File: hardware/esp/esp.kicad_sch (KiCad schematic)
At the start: 34 parts, among them J1 USB_C_Receptacle_USB2.0_16P, J2 Conn_01x02, J3 USB_C_Receptacle_USB2.0_16P, J4 Conn_01x02, SW1 RESET, SW2 BOOT, U1 AMS1117-3.3, U2 ESP32-S3-WROOM-1, U6 CP2102N-Axx-xQFN20

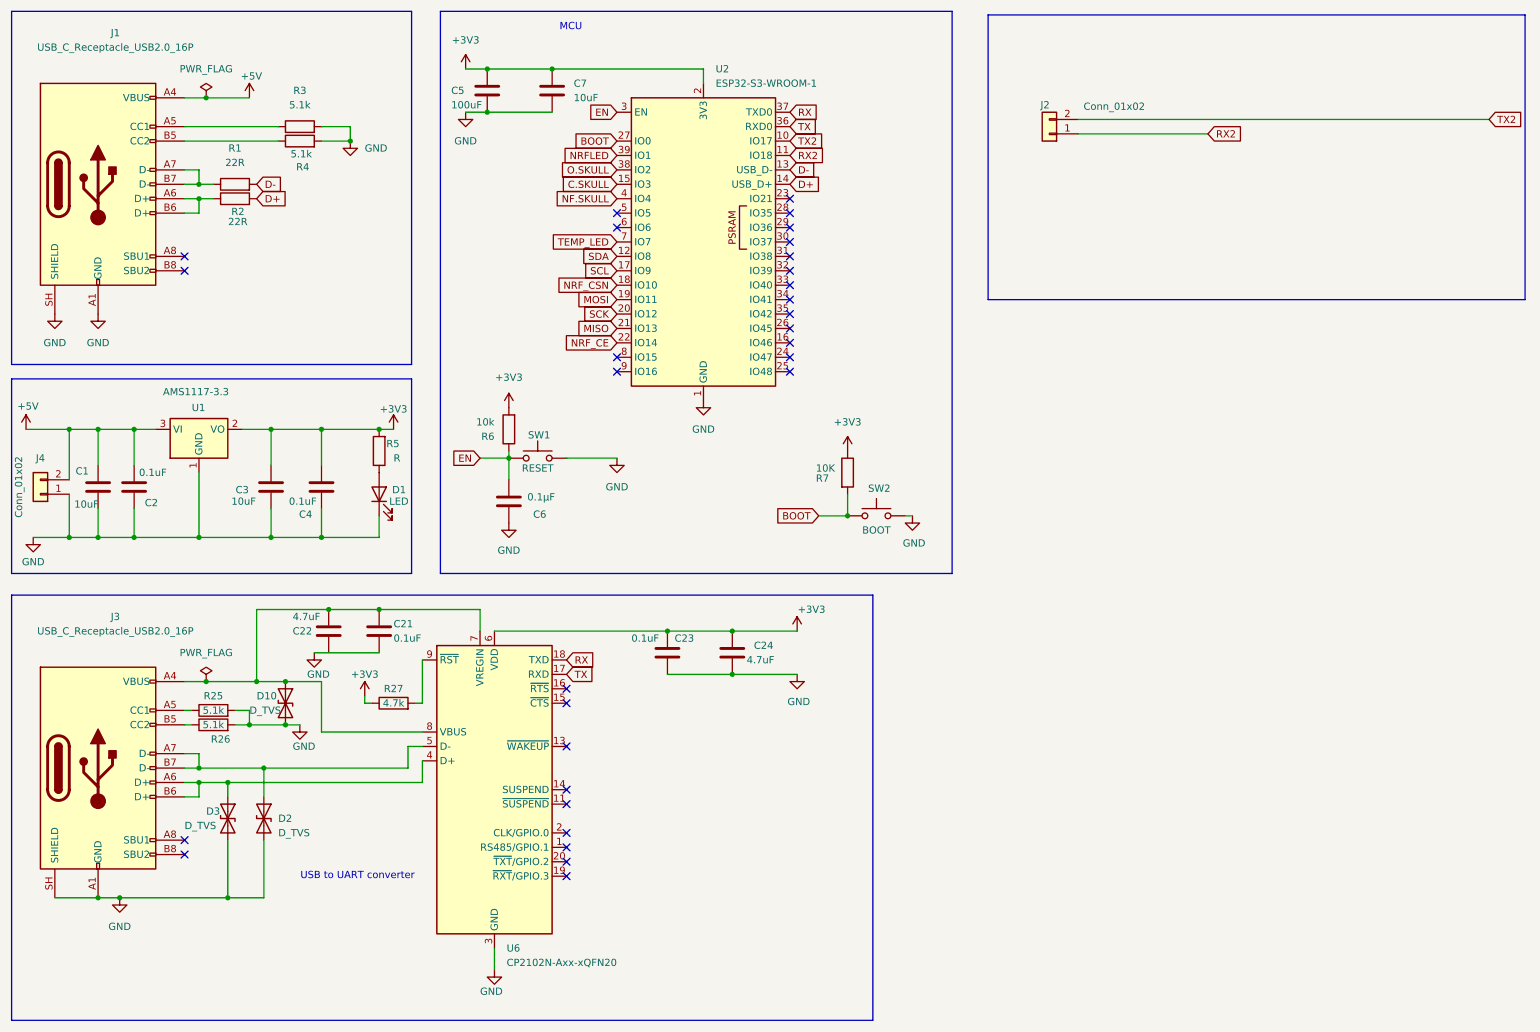
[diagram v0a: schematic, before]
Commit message: Updating pins, and scehmatic
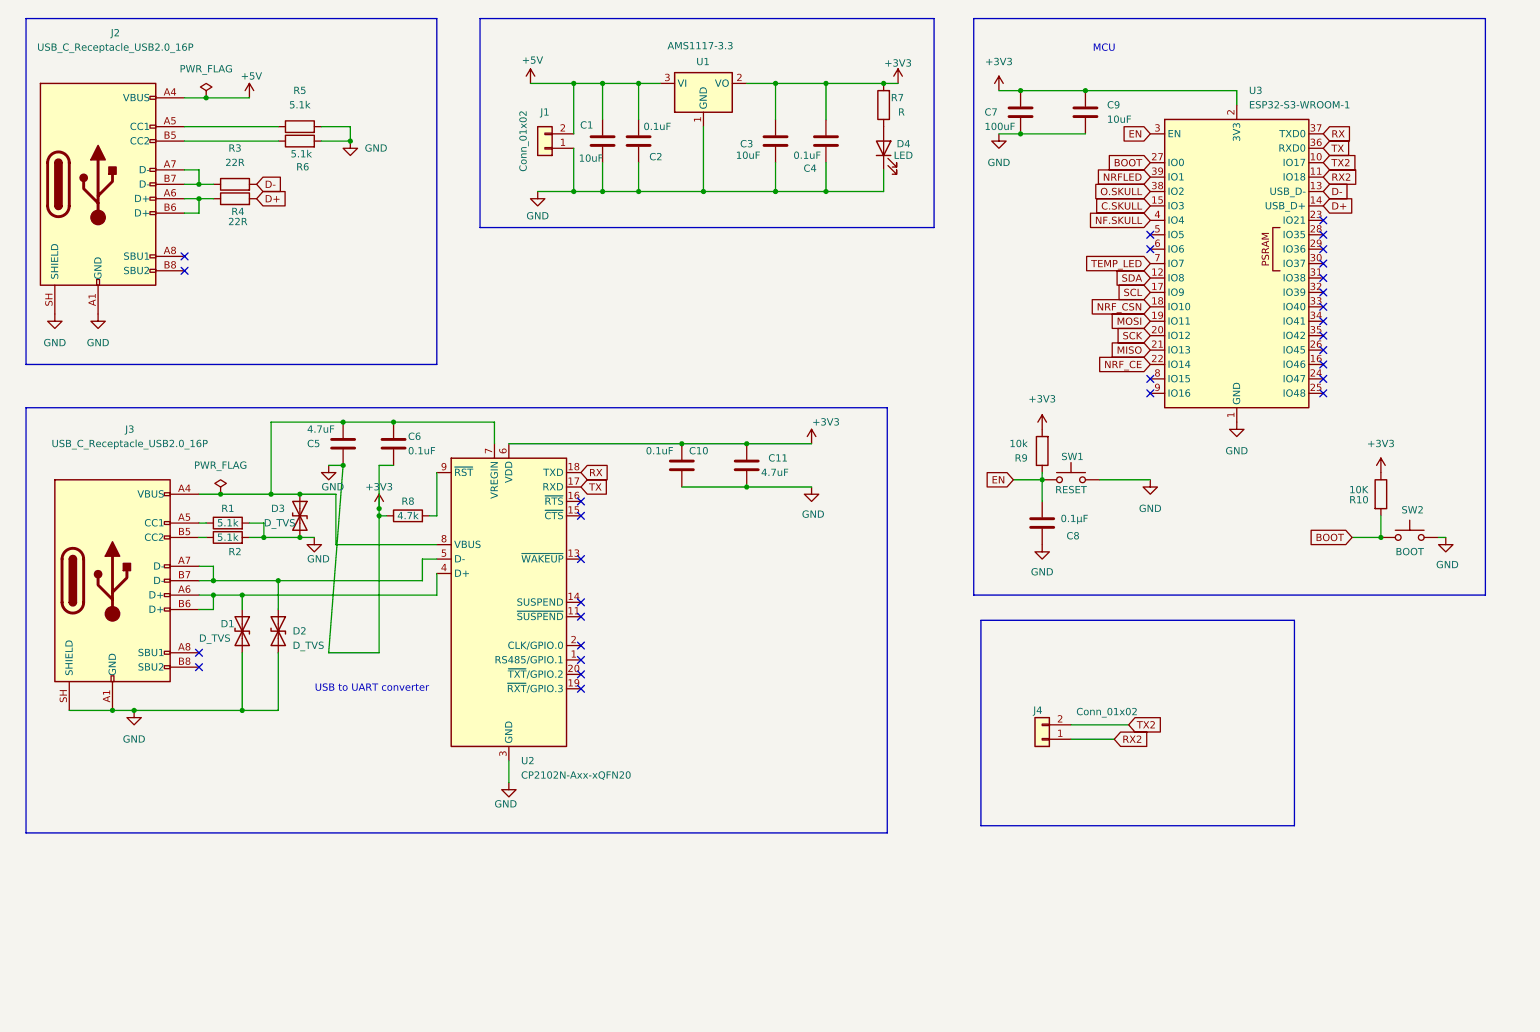
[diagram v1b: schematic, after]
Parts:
- renumbered C23 to C10, C24 to C11, C22 to C5, C21 to C6, C5 to C7, C6 to C8, C7 to C9, D3 to D1, D10 to D3, D1 to D4, J4 to J1, J1 to J2, J2 to J4, R25 to R1, R7 to R10, R26 to R2, R1 to R3, R2 to R4, R3 to R5, R4 to R6, R5 to R7, R27 to R8, R6 to R9, U6 to U2, U2 to U3
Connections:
- net GND is gone; now on net +3V3: C1.2, C10.2, C11.2, C2.2, C3.2, C4.2, C6.2, C7.1, C8.1, C9.1, D1.2 (A2), D2.2 (A2), D3.2 (A2), D4.1 (K), J1.1 (Pin_1), J2.A1 (GND), J2.A12 (GND), J2.B1 (GND), J2.B12 (GND), J2.SH (SHIELD), J3.A1 (GND), J3.A12 (GND), J3.B1 (GND), J3.B12 (GND), J3.SH (SHIELD), R1.2, R2.2, R5.2, R6.2, SW1.2, SW2.2, U1.1 (GND), U2.12 (GND), U2.21 (GND), U2.3 (GND), U3.1 (GND), U3.40 (GND), U3.41 (GND)
- net +3V3: now also C5.2
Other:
- moved on the sheet: C1, C10, C11, C2, C3, C4, C5, C6, C7, C8, C9, D1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
